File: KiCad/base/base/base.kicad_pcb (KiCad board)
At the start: 2 copper layers, 133.6 x 74.9 mm, 2 parts

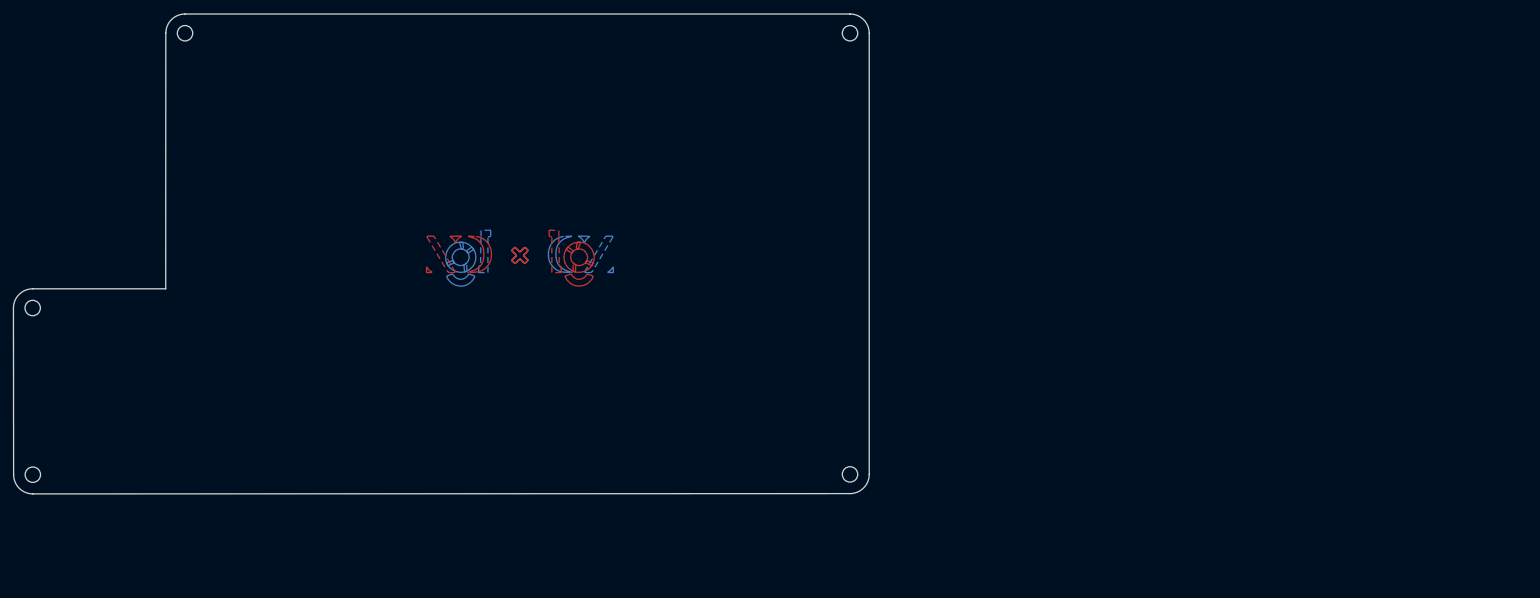
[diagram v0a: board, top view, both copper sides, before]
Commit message: various fixes and changes
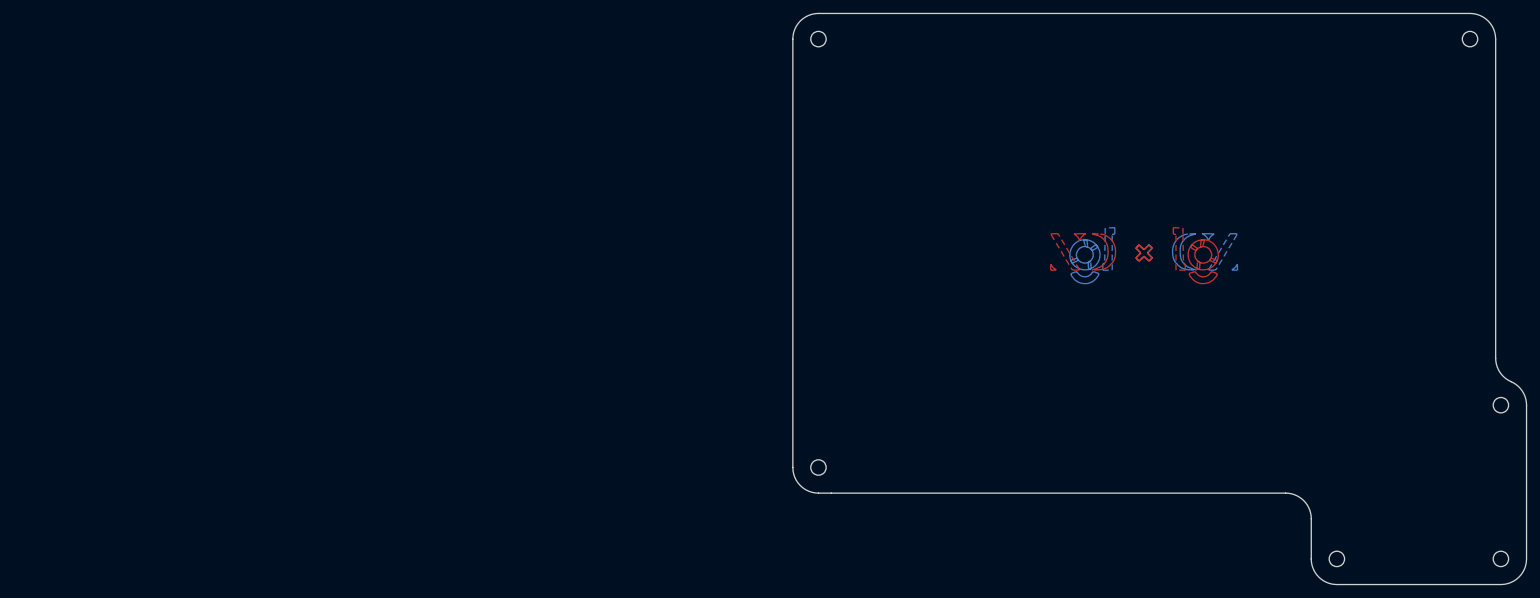
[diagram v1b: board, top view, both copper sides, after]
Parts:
- moved G*** 97.4 mm to (193.8, 87.8)
- moved G*** 97.4 mm to (196.8, 87.8)
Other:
- board size 133.6 x 74.9 mm -> 114.5 x 89.1 mm
